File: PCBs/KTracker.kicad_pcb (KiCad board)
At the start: 2 copper layers, 49.9 x 20.6 mm, 44 parts, among them J1 Conn_01x02_Female, J2 Conn_01x04_Female, P1 USB_C_Plug_USB2.0, SW1 Option/FLASH Switch, SW3 SW_SPDT MAIN POWER, U1 ME6211C, U2 TP4056, U6 ESP-12F, U7 CH340C, U9 MPU-9250

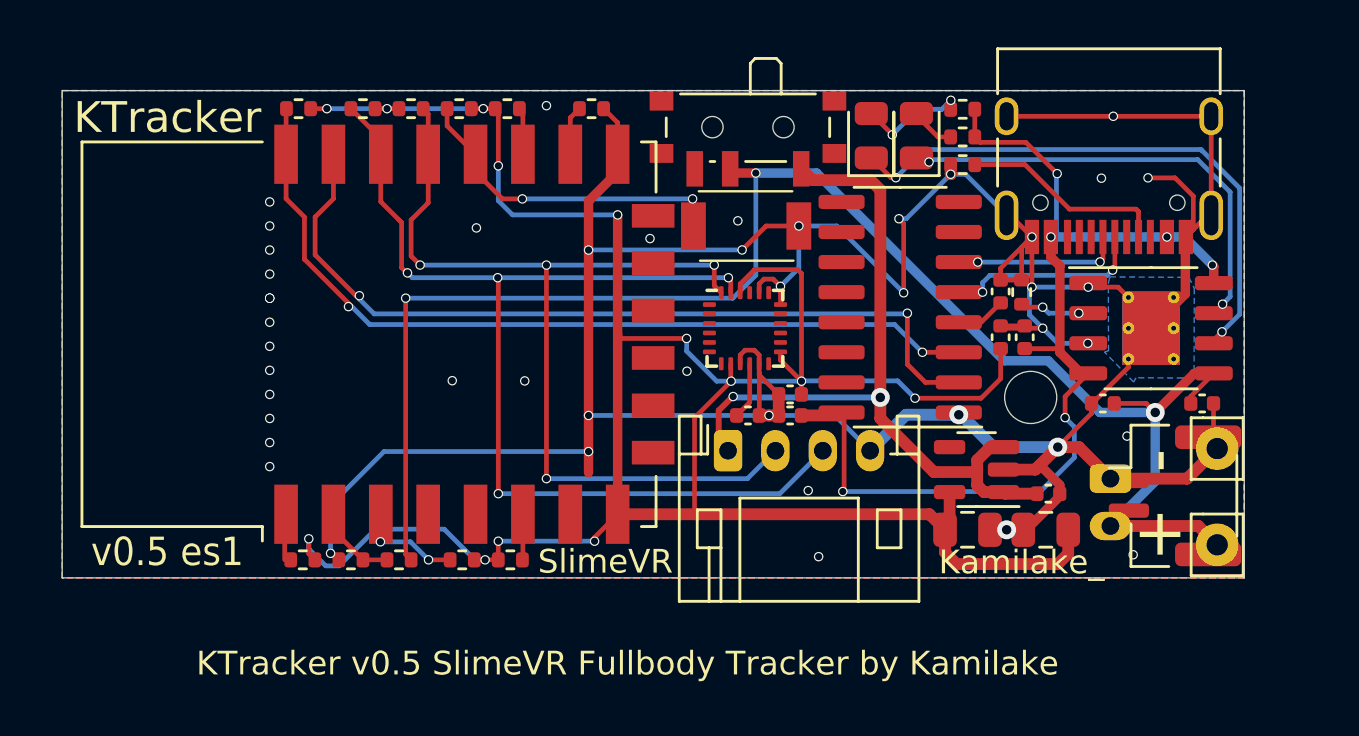
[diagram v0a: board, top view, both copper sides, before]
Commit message: .
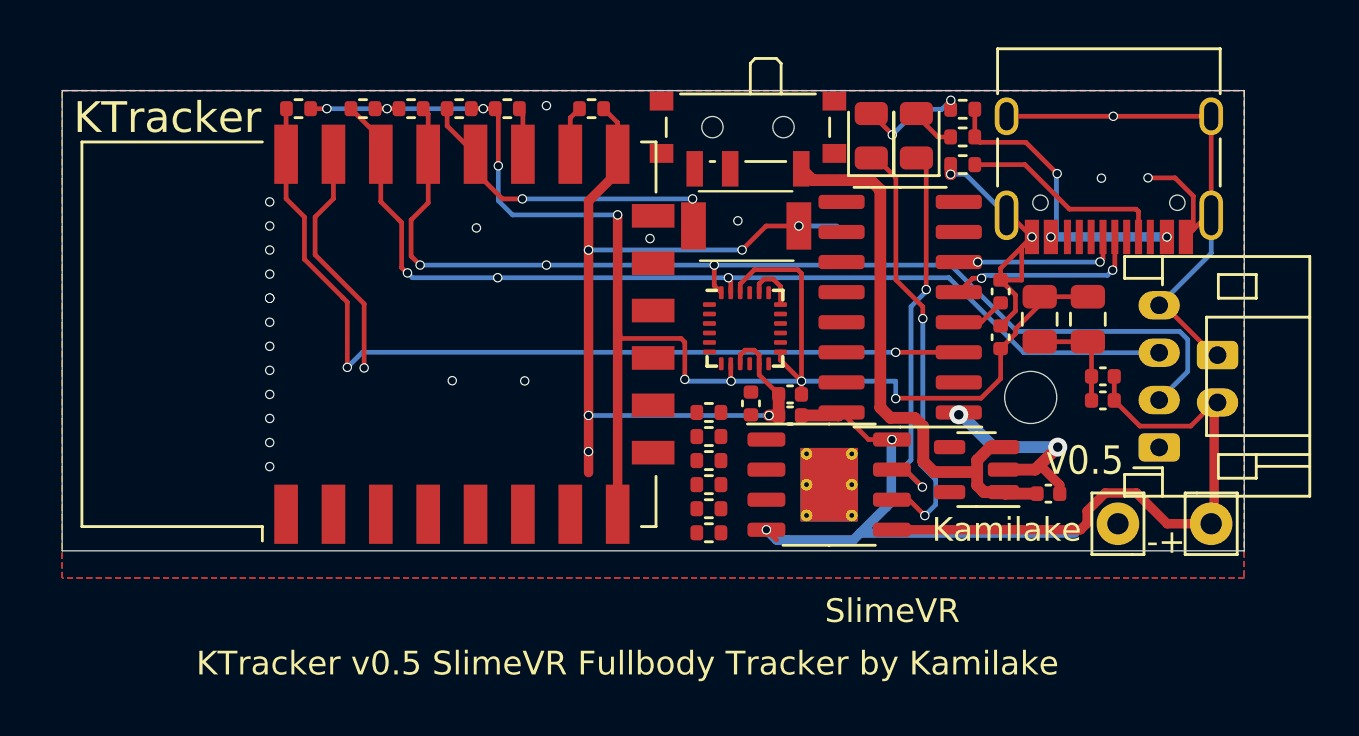
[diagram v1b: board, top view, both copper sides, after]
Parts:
- removed C1: 10uF, Capacitor_SMD:C_0402_1005Metric
- removed JST-MP: JST_GH_BM02B-GHS-TBT_1x02-1MP_P1.25mm_Vertical, Connector_JST:JST_GH_BM02B-GHS-TBT_1x02-1MP_P1.25mm_Vertical
- moved J2 18.2 mm to (136.5, 70.8), turned to 90 degrees
- moved R8 17.2 mm to (117.5, 74.4)
- moved R14 16.0 mm to (117.5, 70.4), turned to 180 degrees
- moved U2 15.1 mm to (122.6, 72.4)
- moved R4 14.2 mm to (117.5, 69.3), turned to 0 degrees
- moved R13 13.7 mm to (117.5, 71.4)
- moved R2 10.6 mm to (117.5, 73.4)
- moved C19 9.40 mm to (131.4, 65.4), turned to -90 degrees
- moved C20 9.07 mm to (133.5, 65.4), turned to -90 degrees
- moved R17 8.96 mm to (117.5, 72.4), turned to 180 degrees
- moved J1 6.90 mm to (139.0, 66.9)
- moved TP2 5.26 mm to (134.7, 74.0), turned to 90 degrees
- moved C10 4.19 mm to (134.1, 68.8), turned to 180 degrees
- moved C13 1.14 mm to (134.1, 67.8)
- moved TP1 0.92 mm to (138.7, 74.0)
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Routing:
- net GND: track 154.2 -> 95.1 mm, vias 46 -> 32
- net BATT+: track 70.0 -> 26.2 mm, vias 3 -> 0
- net +3V3: track 108.4 -> 67.0 mm, vias 13 -> 9
- net UART_ESP-: track 35.3 -> 10.3 mm, vias 2 -> 1
- net VBAT: track 32.4 -> 24.1 mm, vias 2 -> 0
- net VBUS: track 44.0 -> 36.2 mm, vias 6 -> 5
- net Net-(D2-Pad1): track 23.9 -> 18.3 mm
- net SDA: track 40.0 -> 45.2 mm, vias 4 -> 3
- net Net-(R2-Pad2): track 4.43 -> 0.00 mm, vias 2 -> 0
- net SCL: track 45.8 -> 41.7 mm, vias 4 -> 3
- net ADC: track 3.45 -> 0.00 mm
- net Net-(R4-Pad1): track 2.97 -> 0.00 mm, vias 2 -> 0
- net Net-(D1-Pad1): track 19.7 -> 17.1 mm
- net Net-(C7-Pad1): track 2.42 -> 0.00 mm
- net UART_ESP+: track 36.2 -> 38.4 mm
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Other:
- board size 49.9 x 20.6 mm -> 49.9 x 19.4 mm
- board text added: "-+"
- board text added: "Kamilake"
- board text added: "v0.5"
- board text removed: "+"
- board text removed: "-"
- board text removed: "Kamilake_"
- board text removed: "v0.5 es1"
